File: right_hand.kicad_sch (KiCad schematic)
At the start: 2 parts, among them J1 USB_C_Receptacle_USB2.0_16P

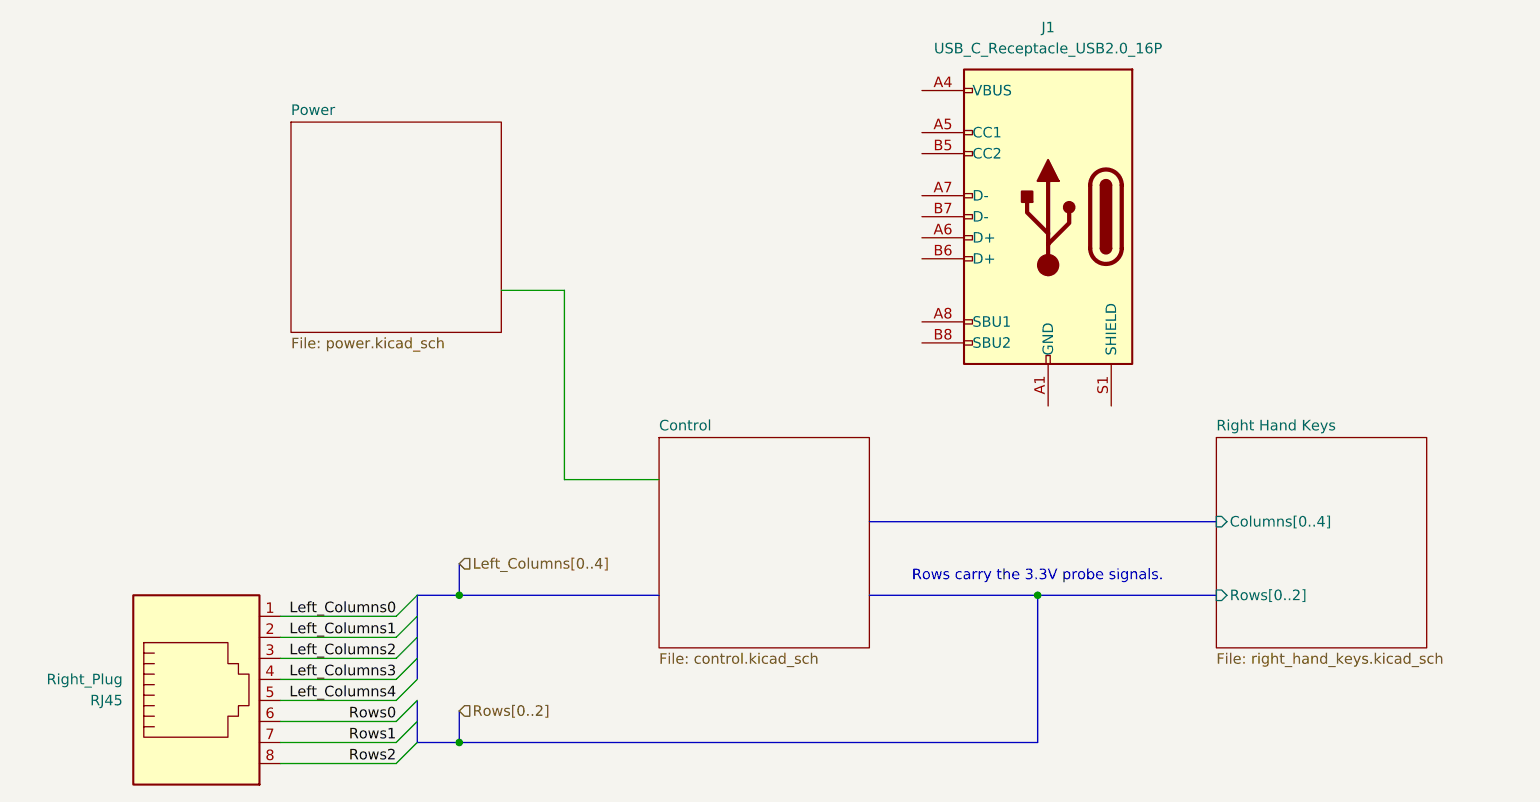
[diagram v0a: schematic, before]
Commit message: Design power
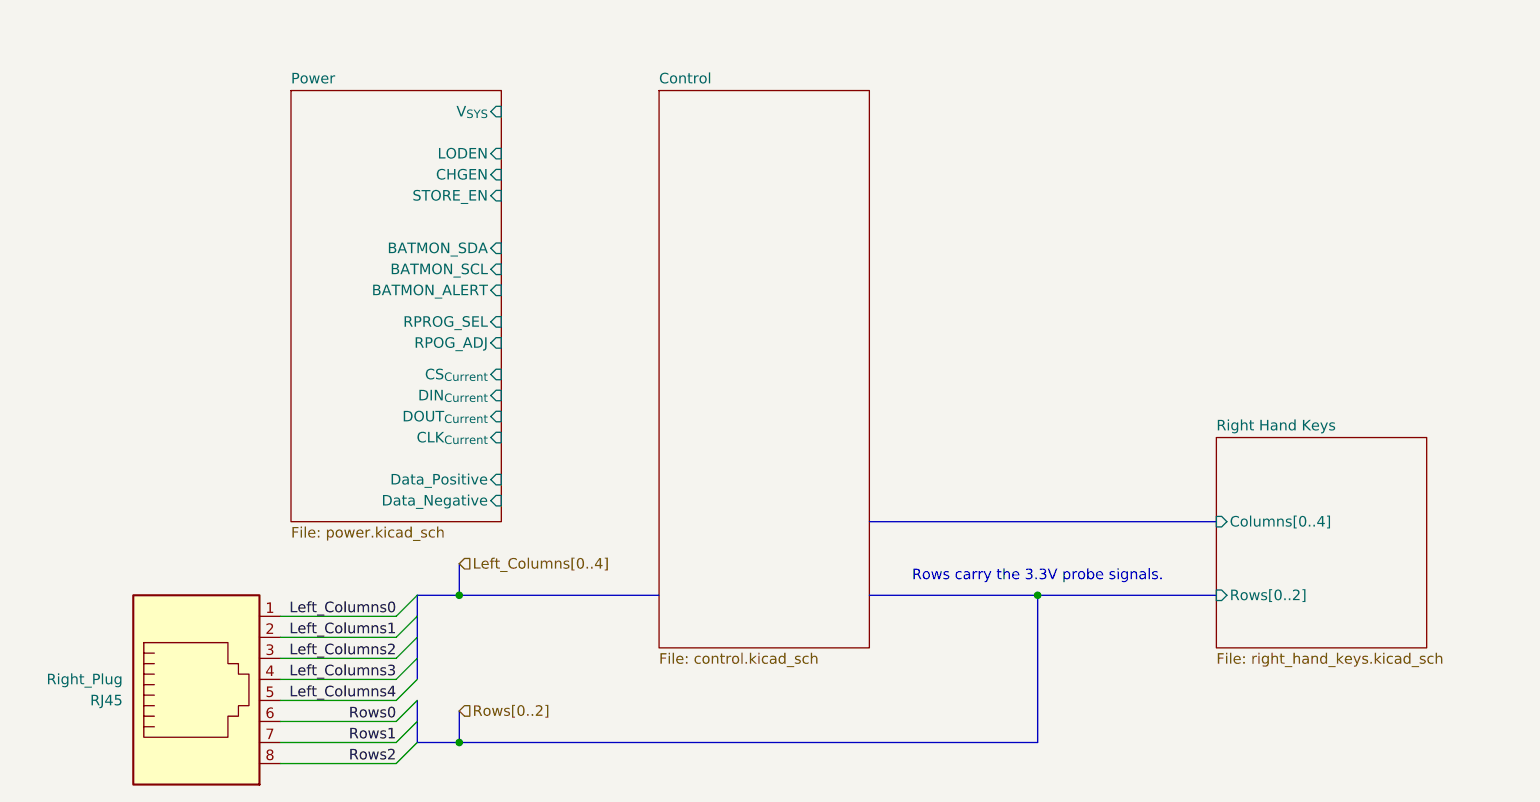
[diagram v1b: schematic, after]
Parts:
- removed J1: USB_C_Receptacle_USB2.0_16P, symbol Connector:USB_C_Receptacle_USB2.0_16P
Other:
- sheet Power ports: added BATMON_ALERT, BATMON_SCL, BATMON_SDA, CHGEN, CLK_{Current}, CS_{Current}, DIN_{Current}, DOUT_{Current}, Data_Negative, Data_Positive, LODEN, RPOG_ADJ, RPROG_SEL, STORE_EN, V_{SYS}; removed none
- title: Port Plover -> Stenoswitch
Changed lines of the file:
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@@
 	(paper "A5")
 	(title_block
-		(title "Port Plover")
-		(date "2025-07-28")
+		(title "Stenoswitch")
 		(rev "0.1")
 		(company "https://github.com/Bennett-Petzold/port_plover")
@@
 	(wire
 		(pts
-			(xy 81.28 69.85) (xy 92.71 69.85)
-		)
-		(stroke
-			(width 0)
-			(type default)
-		)
-	)
-	(wire
-		(pts
 			(xy 60.96 104.14) (xy 46.99 104.14)
 		)
@@
 	(wire
 		(pts
-			(xy 73.66 46.99) (xy 81.28 46.99)
-		)
-		(stroke
-			(width 0)
-			(type default)
-		)
-	)
-	(wire
-		(pts
 			(xy 60.96 96.52) (xy 46.99 96.52)
-		)
-		(stroke
-			(width 0)
-			(type default)
-		)
-	)
-	(wire
-		(pts
-			(xy 81.28 46.99) (xy 81.28 69.85)
 		)
 		(stroke
@@
 		)
 	)
-	(symbol
-		(lib_id "Connector:USB_C_Receptacle_USB2.0_16P")
-		(at 139.7 38.1 0)
-		(mirror y)
-		(unit 1)
+	(sheet
+		(at 92.71 22.86)
+		(size 25.4 67.31)
 		(exclude_from_sim no)
 		(in_bom yes)
@@
 		(dnp no)
 		(fields_autoplaced yes)
-		(property "Reference" "J1"
-			(at 139.7 15.24 0)
-			(effects
-				(font
-					(size 1.27 1.27)
-				)
-			)
-		)
-		(property "Value" "USB_C_Receptacle_USB2.0_16P"
-			(at 139.7 17.78 0)
-			(effects
-				(font
-					(size 1.27 1.27)
-				)
-			)
-		)
-		(property "Footprint" ""
-			(at 135.89 38.1 0)
-			(effects
-				(font
-					(size 1.27 1.27)
-				)
-				(hide yes)
-			)
-		)
-		(property "Datasheet" "https://www.usb.org/sites/default/files/documents/usb_type-c.zip"
-			(at 135.89 38.1 0)
-			(effects
-				(font
-					(size 1.27 1.27)
-				)
-				(hide yes)
-			)
-		)
-		(property "Description" "USB 2.0-only 16P Type-C Receptacle connector"
-			(at 139.7 38.1 0)
-			(effects
-				(font
-					(size 1.27 1.27)
-				)
-				(hide yes)
-			)
-		)
-		(pin "A5"
-		)
-		(pin "A8"
-		)
-		(pin "B7"
-		)
-		(pin "A9"
-		)
-		(pin "B1"
-		)
-		(pin "A4"
-		)
-		(pin "B12"
-		)
-		(pin "A1"
-		)
-		(pin "B5"
-		)
-		(pin "A12"
-		)
-		(pin "B6"
-		)
-		(pin "A7"
-		)
-		(pin "S1"
-		)
-		(pin "A6"
-		)
-		(pin "B9"
-		)
-		(pin "B8"
-		)
-		(pin "B4"
+		(stroke
+			(width 0.1524)
+			(type solid)
+		)
+		(fill
+			(color 0 0 0 0.0000)
+		)
+		(property "Sheetname" "Control"
+			(at 92.71 22.1484 0)
+			(effects
+				(font
+					(size 1.27 1.27)
+				)
+				(justify left bottom)
+			)
+		)
+		(property "Sheetfile" "control.kicad_sch"
+			(at 92.71 90.7546 0)
+			(effects
+				(font
+					(size 1.27 1.27)
+				)
+				(justify left top)
+			)
 		)
 		(instances
-			(project ""
+			(project "portable_steno"
 				(path "/06a6eca0-edda-4cc0-a23f-017602e67f07/99f3b279-b2b0-4dd5-ab05-9b518546ce95"
-					(reference "J1")
-					(unit 1)
+					(page "6")
 				)
 			)
@@
 	)
 	(sheet
-		(at 92.71 64.77)
-		(size 25.4 25.4)
+		(at 48.26 22.86)
+		(size 25.4 52.07)
 		(exclude_from_sim no)
 		(in_bom yes)
@@
 			(color 0 0 0 0.0000)
 		)
-		(property "Sheetname" "Control"
-			(at 92.71 64.0584 0)
+		(property "Sheetname" "Power"
+			(at 48.26 22.1484 0)
 			(effects
 				(font
@@
 			)
 		)
-		(property "Sheetfile" "control.kicad_sch"
-			(at 92.71 90.7546 0)
+		(property "Sheetfile" "power.kicad_sch"
+			(at 48.26 75.5146 0)
 			(effects
 				(font
@@
 			)
 		)
-		(instances
-			(project "portable_steno"
-				(path "/06a6eca0-edda-4cc0-a23f-017602e67f07/99f3b279-b2b0-4dd5-ab05-9b518546ce95"
-					(page "6")
-				)
-			)
-		)
-	)
-	(sheet
-		(at 48.26 26.67)
-		(size 25.4 25.4)
-		(exclude_from_sim no)
-		(in_bom yes)
-		(on_board yes)
-		(dnp no)
-		(fields_autoplaced yes)
-		(stroke
-			(width 0.1524)
-			(type solid)
-		)
-		(fill
-			(color 0 0 0 0.0000)
-		)
-		(property "Sheetname" "Power"
-			(at 48.26 25.9584 0)
-			(effects
-				(font
-					(size 1.27 1.27)
-				)
-				(justify left bottom)
-			)
-		)
-		(property "Sheetfile" "power.kicad_sch"
-			(at 48.26 52.6546 0)
-			(effects
-				(font
-					(size 1.27 1.27)
-				)
-				(justify left top)
-			)
-		)
+		(pin "Data_Negative" input
+			(at 73.66 72.39 0)
+			(effects
+				(font
+					(size 1.27 1.27)
+				)
+				(justify right)
+			)
+		)
+		(pin "Data_Positive" input
+			(at 73.66 69.85 0)
+			(effects
+				(font
+					(size 1.27 1.27)
+				)
+				(justify right)
+			)
+		)
+		(pin "DOUT_{Current}" input
+			(at 73.66 62.23 0)
+			(effects
+				(font
+					(size 1.27 1.27)
+				)
+				(justify right)
+			)
+		)
+		(pin "BATMON_SCL" input
+			(at 73.66 44.45 0)
+			(effects
+				(font
+					(size 1.27 1.27)
+				)
+				(justify right)
+			)
+		)
+		(pin "RPOG_ADJ" input
+			(at 73.66 53.34 0)
+			(effects
+				(font
+					(size 1.27 1.27)
+				)
+				(justify right)
+			)
+		)
+		(pin "RPROG_SEL" input
+			(at 73.66 50.8 0)
+			(effects
+				(font
+					(size 1.27 1.27)
+				)
+				(justify right)
+			)
+		)
+		(pin "CS_{Current}" input
+			(at 73.66 57.15 0)
+			(effects
+				(font
+					(size 1.27 1.27)
+				)
+				(justify right)
+			)
+		)
+		(pin "DIN_{Current}" input
+			(at 73.66 59.69 0)
+			(effects
+				(font
+					(size 1.27 1.27)
+				)
+				(justify right)
+			)
+		)
+		(pin "BATMON_SDA" input
+			(at 73.66 41.91 0)
+			(effects
+				(font
+					(size 1.27 1.27)
+				)
+				(justify right)
+			)
+		)
+		(pin "STORE_EN" input
+			(at 73.66 35.56 0)
+			(effects
+				(font
+					(size 1.27 1.27)
+				)
+				(justify right)
+			)
+		)
+		(pin "CHGEN" input
+			(at 73.66 33.02 0)
+			(effects
+				(font
+					(size 1.27 1.27)
+				)
+				(justify right)
+			)
+		)
+		(pin "V_{SYS}" input
+			(at 73.66 25.4 0)
+			(effects
+				(font
+					(size 1.27 1.27)
+				)
+				(justify right)
+			)
+		)
+		(pin "LODEN" input
+			(at 73.66 30.48 0)
+			(effects
+				(font
+					(size 1.27 1.27)
+				)
+				(justify right)
+			)
+		)
+		(pin "BATMON_ALERT" input
+			(at 73.66 46.99 0)
+			(effects
+				(font
+					(size 1.27 1.27)
+				)
+				(justify right)
+			)
+		)
+		(pin "CLK_{Current}" input
+			(at 73.66 64.77 0)
+			(effects
+				(font
+					(size 1.27 1.27)
+				)
+				(justify right)
+			)
+		)
